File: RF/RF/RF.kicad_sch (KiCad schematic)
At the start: 0 parts

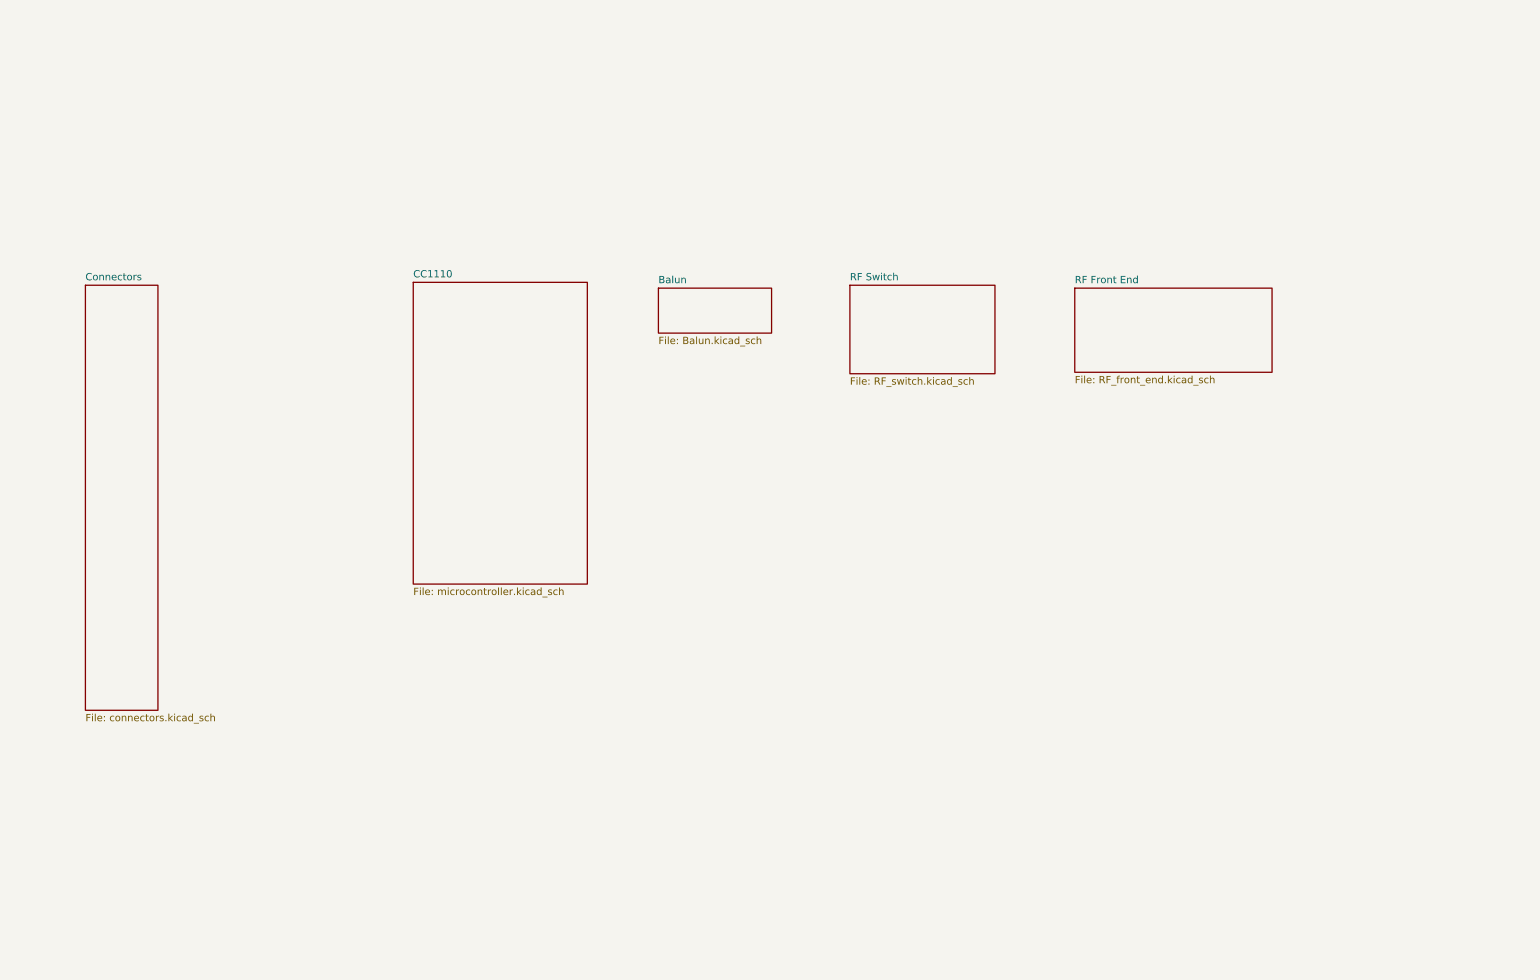
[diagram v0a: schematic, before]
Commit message: added external memory
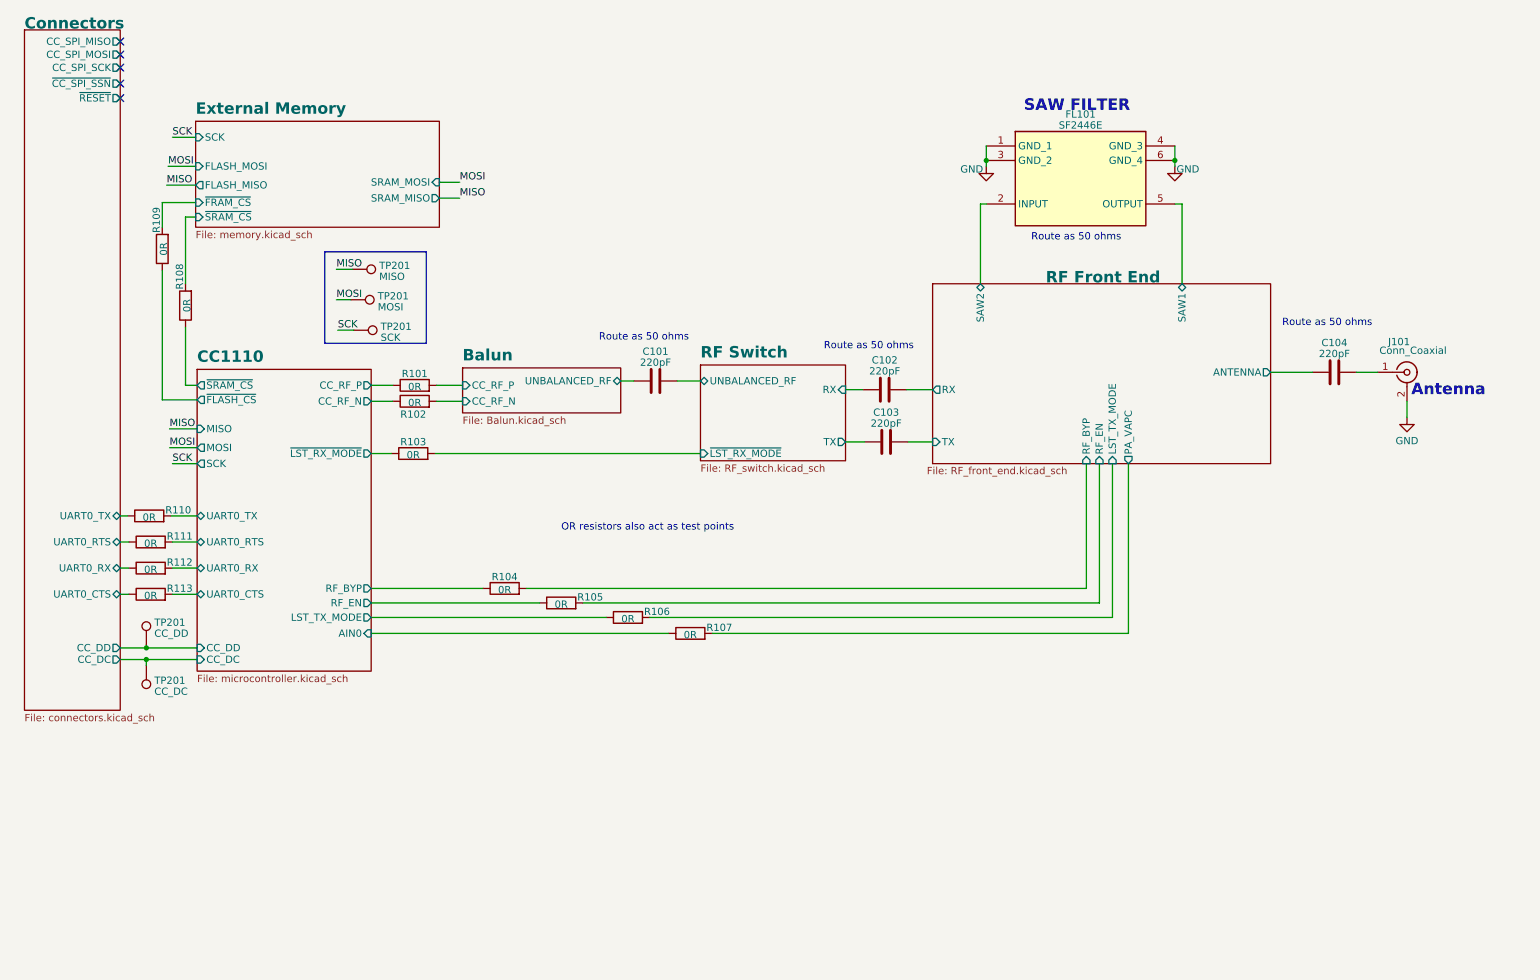
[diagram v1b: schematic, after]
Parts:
- added C101, C102, C103, C104: 220pF, Capacitor_SMD:C_0603_1608Metric_Pad1.08x0.95mm_HandSolder, symbol Device:C
- added FL101: SF2446E, SamacSys_Parts:SF2446E, symbol SamacSys_Parts:SF2446E
- added J101: Conn_Coaxial, Connector_Coaxial:SMA_Amphenol_901-143_Horizontal, symbol Connector:Conn_Coaxial
- added R101, R102, R103, R104, R105, R106, R107, R108, R109, R110, R111, R112, R113: 0R, Resistor_SMD:R_0603_1608Metric_Pad0.98x0.95mm_HandSolder, symbol Device:R
- added TP201: MOSI, TestPoint:TestPoint_Loop_D3.50mm_Drill1.4mm_Beaded, symbol Connector:TestPoint
- added TP201: MISO, TestPoint:TestPoint_Loop_D3.50mm_Drill1.4mm_Beaded, symbol Connector:TestPoint
- added TP201: CC_DC, TestPoint:TestPoint_Loop_D3.50mm_Drill1.4mm_Beaded, symbol Connector:TestPoint
- added TP201: SCK, TestPoint:TestPoint_Loop_D3.50mm_Drill1.4mm_Beaded, symbol Connector:TestPoint
- added TP201: CC_DD, TestPoint:TestPoint_Loop_D3.50mm_Drill1.4mm_Beaded, symbol Connector:TestPoint
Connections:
- new net: C104.2, J101.1 (In)
- new net Balun/CC_RF_N: R102.2
- new net Balun/CC_RF_P: R101.2
- new net Balun/UNBALANCED_RF: C101.1
- new net CC1110/AIN0: R107.1
- new net CC1110/CC_DC: TP201.1
- new net CC1110/CC_DD: TP201.1
- new net CC1110/CC_RF_N: R102.1
- new net CC1110/CC_RF_P: R101.1
- new net CC1110/LST_TX_MODE: R106.1
- new net CC1110/RF_BYP: R104.1
- new net CC1110/RF_EN: R105.1
- new net CC1110/UART0_CTS: R113.2
- new net CC1110/UART0_RTS: R111.2
- new net CC1110/UART0_RX: R112.2
- new net CC1110/UART0_TX: R110.2
- new net CC1110/~{FLASH_CS}: R109.1
- new net CC1110/~{LST_RX_MODE}: R103.1
- new net CC1110/~{SRAM_CS}: R108.1
- new net Connectors/UART0_CTS: R113.1
- new net Connectors/UART0_RTS: R111.1
- new net Connectors/UART0_RX: R112.1
- new net Connectors/UART0_TX: R110.1
- new net External Memory/~{FRAM_CS}: R109.2
- new net External Memory/~{SRAM_CS}: R108.2
- new net GND: FL101.1 (GND_1), FL101.3 (GND_2), FL101.4 (GND_3), FL101.6 (GND_4), J101.2 (Ext)
- new net MISO: TP201.1
- new net MOSI: TP201.1
- new net RF Front End/ANTENNA: C104.1
- new net RF Front End/LST_TX_MODE: R106.2
- new net RF Front End/PA_VAPC: R107.2
- new net RF Front End/RF_BYP: R104.2
- new net RF Front End/RF_EN: R105.2
- new net RF Front End/RX: C102.2
- new net RF Front End/SAW1: FL101.5 (OUTPUT)
- new net RF Front End/SAW2: FL101.2 (INPUT)
- new net RF Front End/TX: C103.2
- new net RF Switch/RX: C102.1
- new net RF Switch/TX: C103.1
- new net RF Switch/UNBALANCED_RF: C101.2
- new net RF Switch/~{LST_RX_MODE}: R103.2
- new net SCK: TP201.1
- no-connect marks 0 -> 5
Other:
- added sheet External Memory (memory.kicad_sch)
- sheet Balun ports: added CC_RF_N, CC_RF_P, UNBALANCED_RF; removed none
- sheet CC1110 ports: added AIN0, CC_DC, CC_DD, CC_RF_N, CC_RF_P, LST_TX_MODE, MISO, MOSI, RF_BYP, RF_EN, SCK, UART0_CTS, UART0_RTS, UART0_RX, UART0_TX, ~{FLASH_CS}, ~{LST_RX_MODE}, ~{SRAM_CS}; removed none
- sheet Connectors ports: added CC_DC, CC_DD, CC_SPI_MISO, CC_SPI_MOSI, CC_SPI_SCK, UART0_CTS, UART0_RTS, UART0_RX, UART0_TX, ~{CC_SPI_SSN}, ~{RESET}; removed none
- sheet RF Front End ports: added ANTENNA, LST_TX_MODE, PA_VAPC, RF_BYP, RF_EN, RX, SAW1, SAW2, TX; removed none
- sheet RF Switch ports: added RX, TX, UNBALANCED_RF, ~{LST_RX_MODE}; removed none
- note added: "Antenna"
- note added: "OR resistors also act as test points"
- note added: "Route as 50 ohms"
- note added: "SAW FILTER"

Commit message: RF: Push for schematic capture review version 1.0
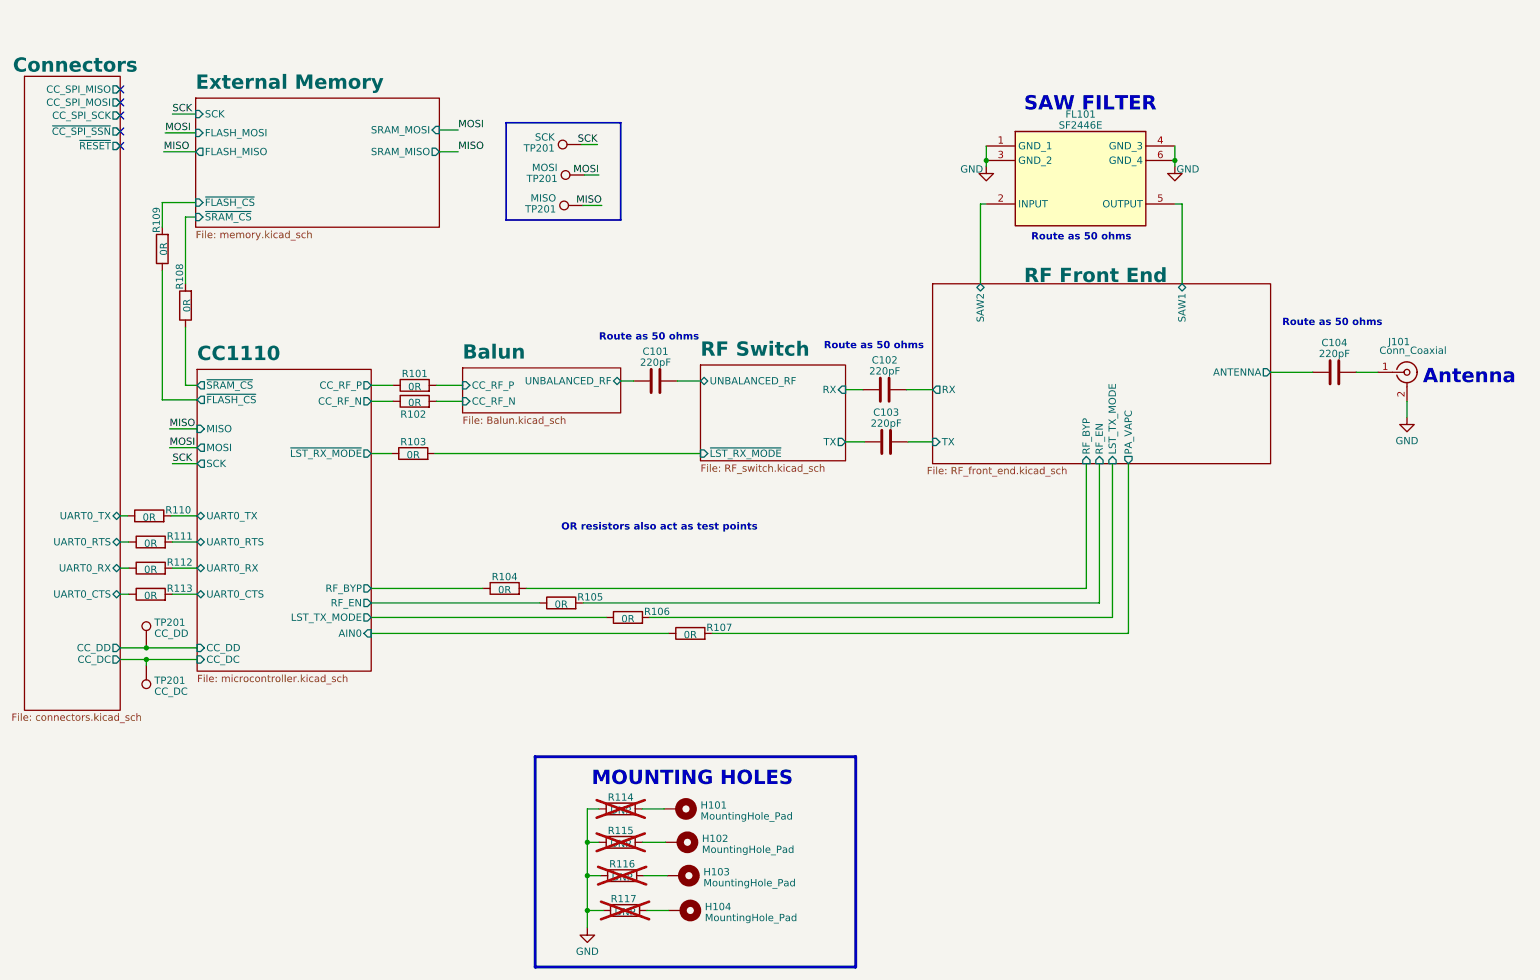
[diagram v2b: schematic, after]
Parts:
- added H101, H102, H103, H104: MountingHole_Pad, MountingHole:MountingHole_2.2mm_M2_DIN965_Pad, symbol Mechanical:MountingHole_Pad
- added R114, R115, R116, R117: DNP, Resistor_SMD:R_0603_1608Metric_Pad0.98x0.95mm_HandSolder, symbol Device:R
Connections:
- net GND: now also R114.1, R115.1, R116.1, R117.1
- net External Memory/~{FRAM_CS} renamed External Memory/~{FLASH_CS}
- new net: H101.1, R114.2
- new net: H103.1, R116.2
- new net: H102.1, R115.2
- new net: H104.1, R117.2
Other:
- sheet External Memory ports: added ~{FLASH_CS}; removed ~{FRAM_CS}
- note added: "MOUNTING HOLES"
- moved on the sheet: TP201
